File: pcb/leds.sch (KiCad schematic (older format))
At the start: 15 parts

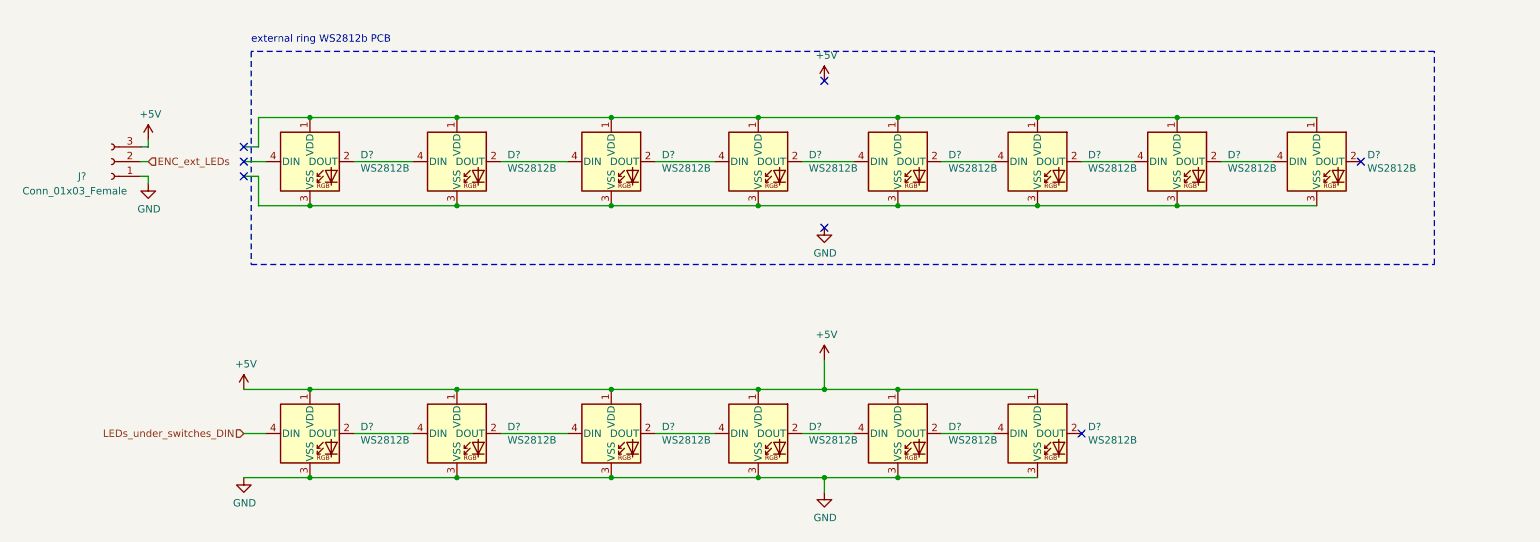
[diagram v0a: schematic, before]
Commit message: Schematic version 1.0
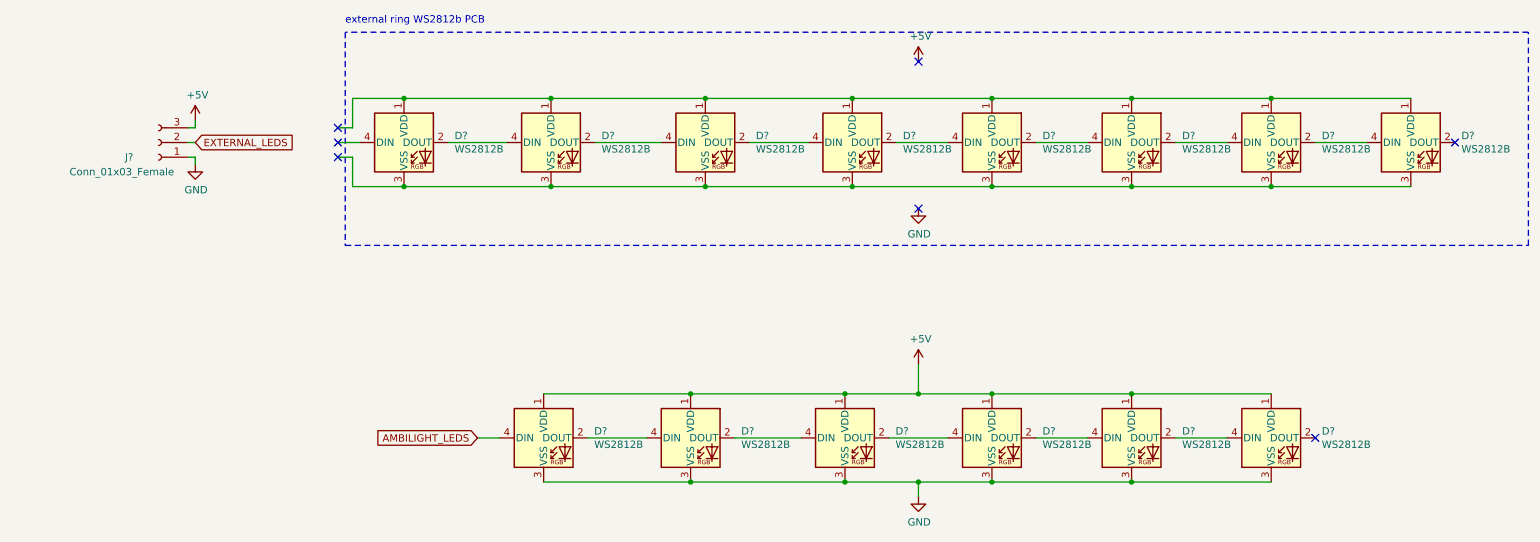
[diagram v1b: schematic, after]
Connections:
- net ENC_ext_LEDs renamed EXTERNAL_LEDS
- net LEDs_under_switches_DIN renamed AMBILIGHT_LEDS
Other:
- moved on the sheet: D?, J?
